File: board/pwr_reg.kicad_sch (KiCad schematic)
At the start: 49 parts, among them J2 9V-30VDC, Q1 IRF9540N, Q2 2N3906, Q3 IRF9540N, Q4 2N3906, SW1 On/Off, SW2 RESET, U1 LM350, U2 LM350, U3 LM350

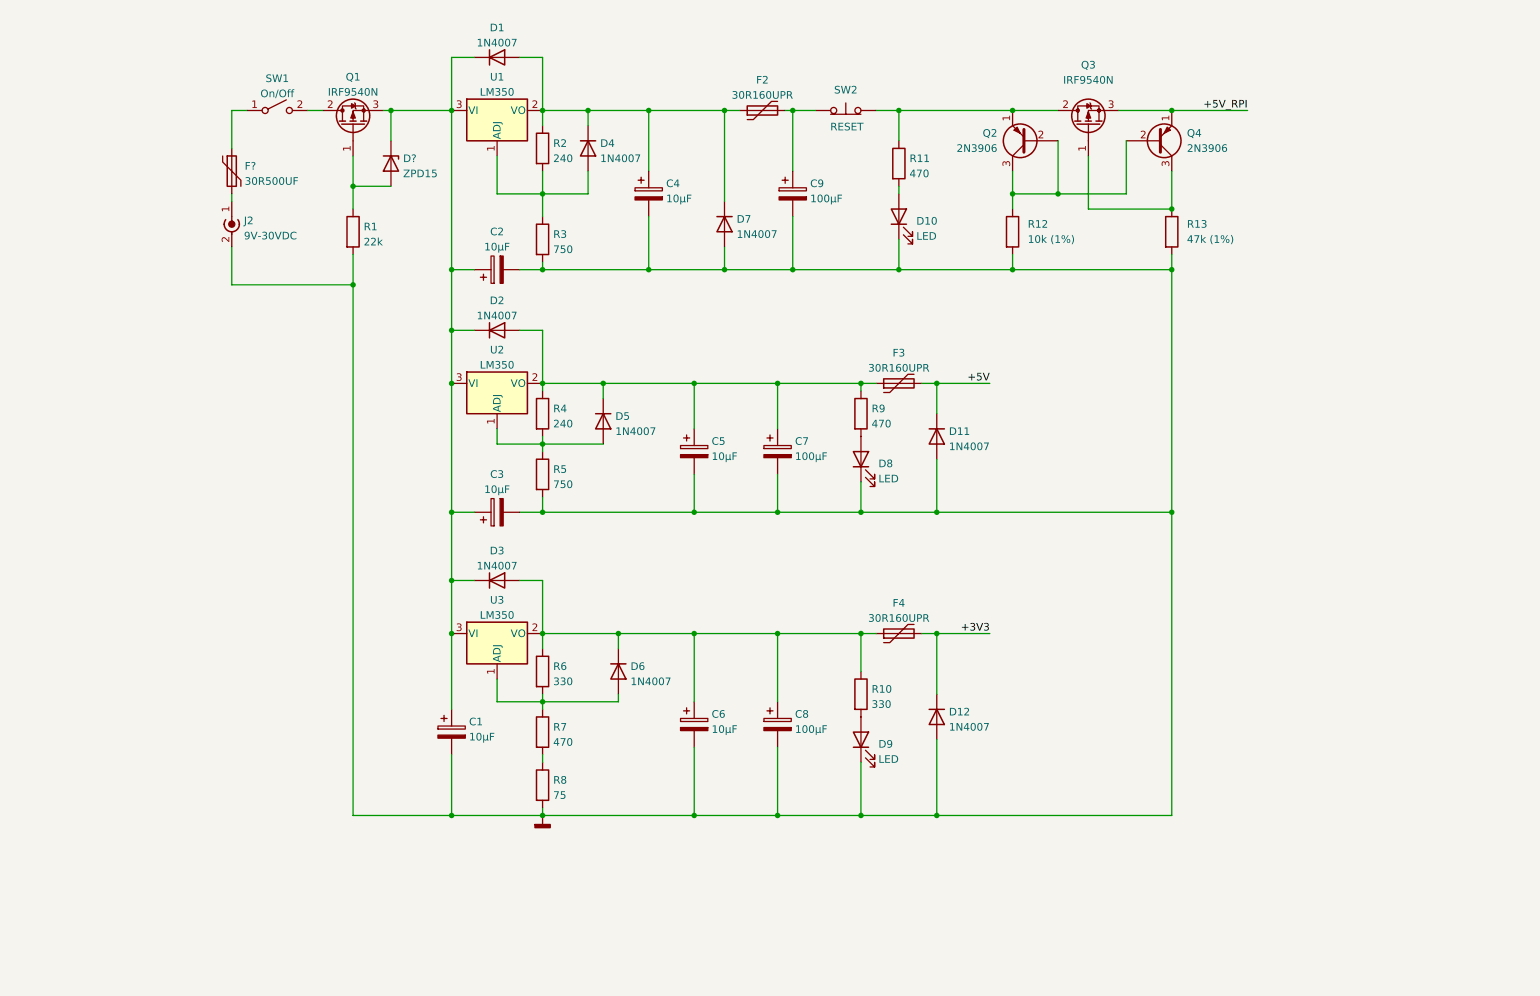
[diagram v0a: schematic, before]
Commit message: Do some cleanup after recent changes.
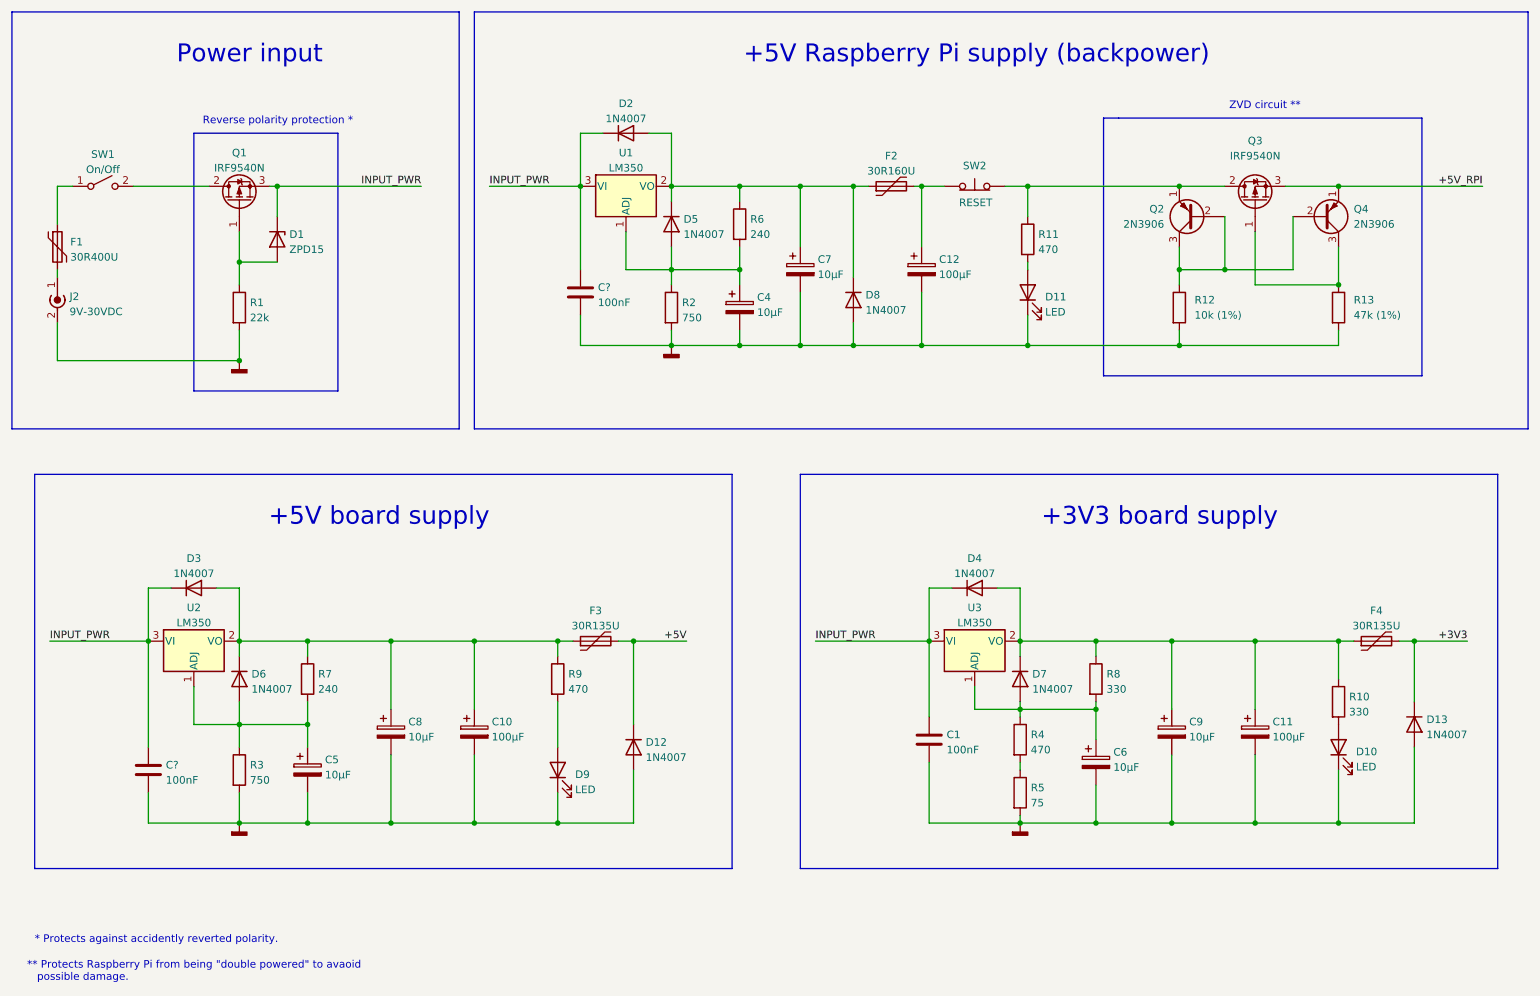
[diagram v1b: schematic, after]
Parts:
- removed C1, C2, C3: 10µF, symbol Device:C_Polarized
- added C1, C? (x2): 100nF, symbol Device:C
- added C4, C5, C6: 10µF, symbol Device:C_Polarized
- F1: renamed from F?; value 30R500UF -> 30R400U; footprint (none) -> Fuse:Fuse_Littelfuse_395Series
- F2: value 30R160UPR -> 30R160U; footprint (none) -> Fuse:Fuse_Littelfuse_395Series
- F3, F4: value 30R160UPR -> 30R135U; footprint (none) -> Fuse:Fuse_Littelfuse_395Series
- J2: footprint (none) -> Connector_Wire:SolderWire-2sqmm_1x02_P7.8mm_D2mm_OD3.9mm
- R1, R10, R11, R12, R13, R9: footprint (none) -> Resistor_THT:R_Axial_DIN0516_L15.5mm_D5.0mm_P7.62mm_Vertical
- R2: renamed from R3; footprint (none) -> Resistor_THT:R_Axial_DIN0516_L15.5mm_D5.0mm_P7.62mm_Vertical
- R3: renamed from R5; footprint (none) -> Resistor_THT:R_Axial_DIN0516_L15.5mm_D5.0mm_P7.62mm_Vertical
- R4: renamed from R7; footprint (none) -> Resistor_THT:R_Axial_DIN0516_L15.5mm_D5.0mm_P7.62mm_Vertical
- R5: renamed from R8; footprint (none) -> Resistor_THT:R_Axial_DIN0516_L15.5mm_D5.0mm_P7.62mm_Vertical
- R6: renamed from R2; footprint (none) -> Resistor_THT:R_Axial_DIN0516_L15.5mm_D5.0mm_P7.62mm_Vertical
- R7: renamed from R4; footprint (none) -> Resistor_THT:R_Axial_DIN0516_L15.5mm_D5.0mm_P7.62mm_Vertical
- R8: renamed from R6; footprint (none) -> Resistor_THT:R_Axial_DIN0516_L15.5mm_D5.0mm_P7.62mm_Vertical
- SW1: footprint (none) -> Connector_Wire:SolderWire-0.5sqmm_1x02_P4.8mm_D0.9mm_OD2.3mm
- gave numbers to parts that had none: 1
- renumbered C7 to C10, C8 to C11, C9 to C12, C4 to C7, C5 to C8, C6 to C9, D9 to D10, D10 to D11, D11 to D12, D12 to D13, D1 to D2, D2 to D3, D3 to D4, D4 to D5, D5 to D6, D6 to D7, D7 to D8, D8 to D9
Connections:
- net GNDD: now also C1.2, C4.2, C5.2, C6.2, C?.2, C?.2
- net INPUT_PWR: now reaches D1.1 (K), D2.1 (K), D3.1 (K), D4.1 (K), Q1.3 (S), U1.3 (VI), U2.3 (VI), U3.3 (VI)
- net INPUT_PWR: now also C1.1, C?.1, C?.1
- net at D7.2 (A), R4.1, R8.2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: now also C6.1
- net at D5.2 (A), R2.1, R6.2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: now also C4.1
- net at D6.2 (A), R3.1, R7.2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: now also C5.1
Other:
- note added: "* Protects against accidently reverted polarity."
- note added: "** Protects Raspberry Pi from being "double powered" to avaoid possible damage."
- note added: "+3V3 board supply"
- note added: "+5V Raspberry Pi supply (backpower)"
- note added: "+5V board supply"
- note added: "Power input"
- note added: "Reverse polarity protection *"
- note added: "ZVD circuit **"
- moved on the sheet: C10, C11, C12, C7, C8, C9, D1, D10, D11, D12, D13, D2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
